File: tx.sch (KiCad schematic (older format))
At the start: 60 parts, among them T2 Transformer_1P_SS, U10 TLV2464CD, U11 SN74CBT3253

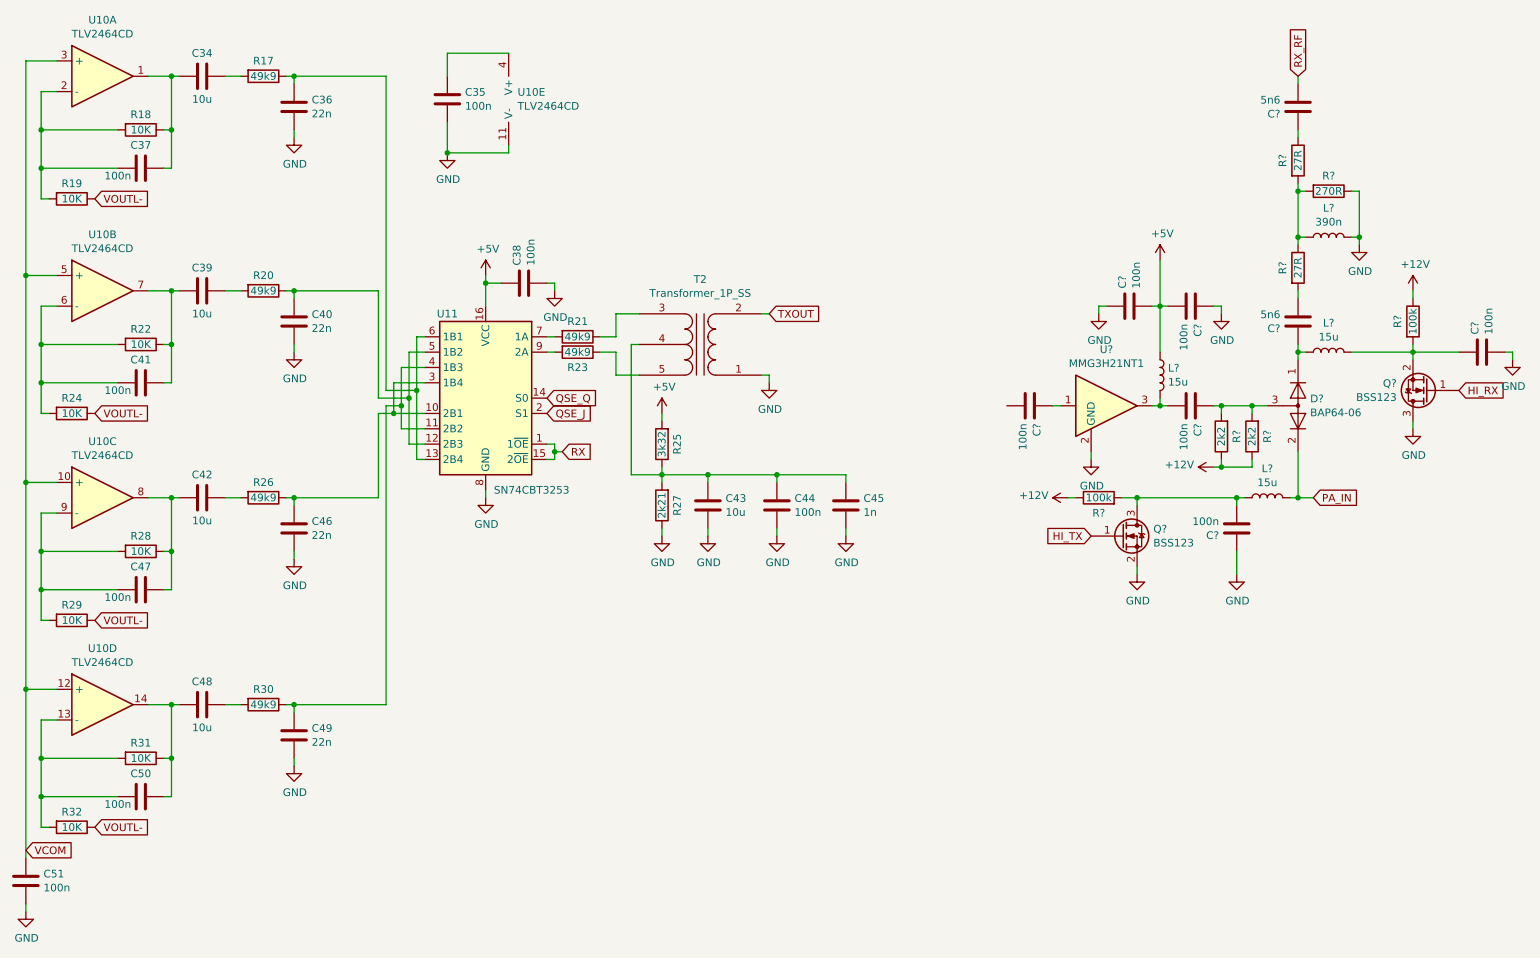
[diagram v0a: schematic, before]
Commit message: First layouting
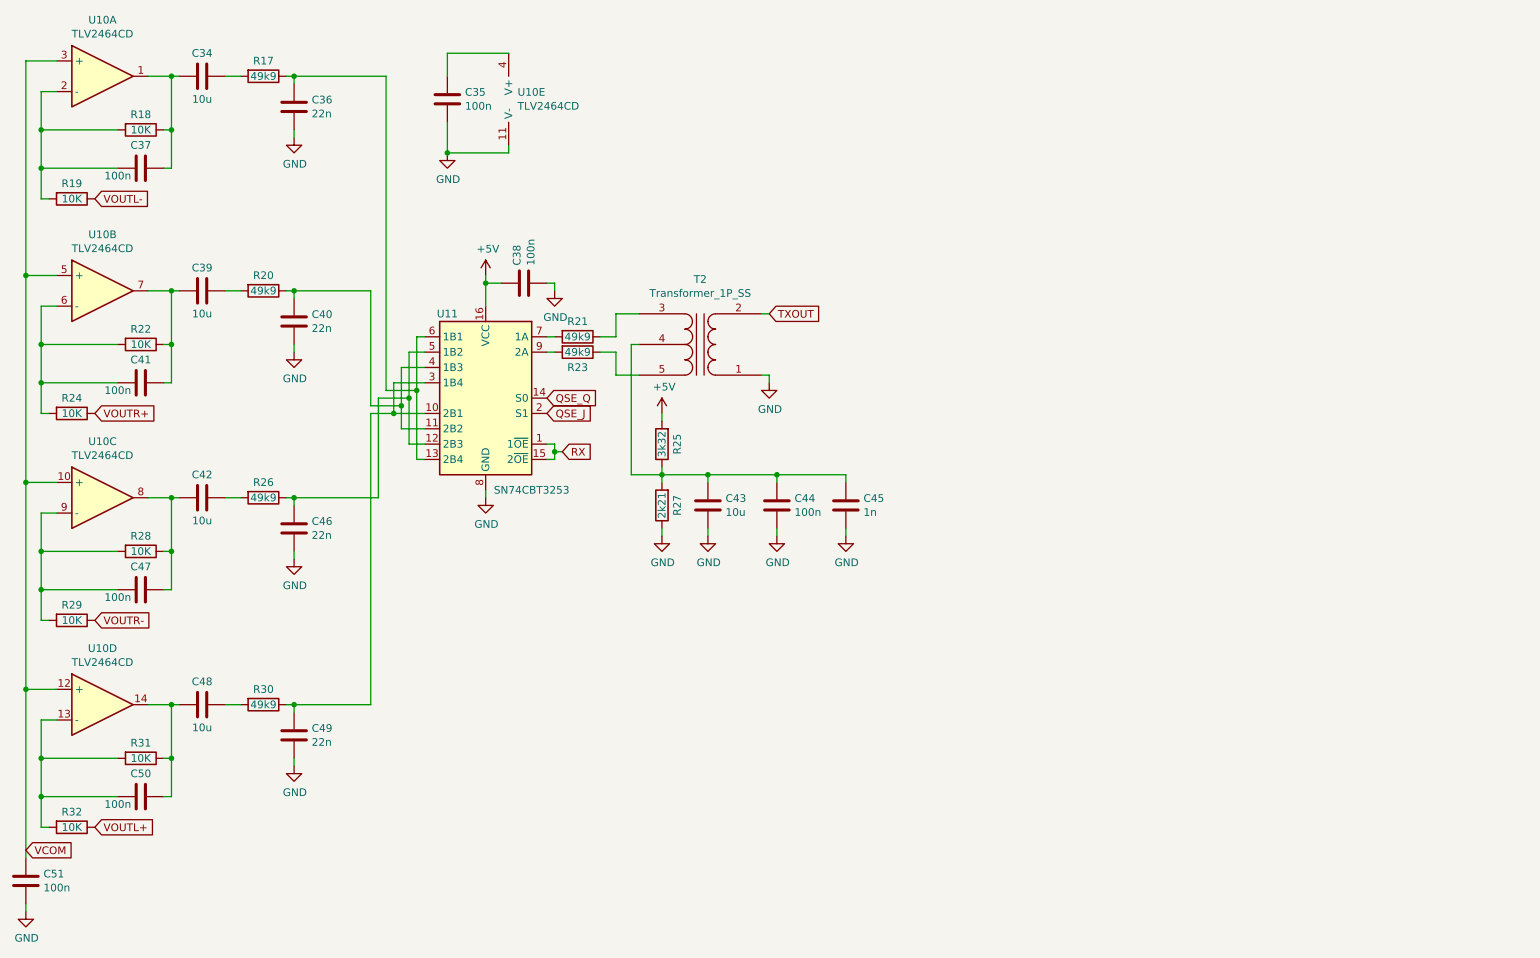
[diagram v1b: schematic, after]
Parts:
- removed C? (x6): 100n, Capacitor_SMD:C_0603_1608Metric, symbol DeltaSDR-rescue:C-Device-DeltaSDR-rescue
- removed C? (x2): 5n6, Capacitor_SMD:C_0603_1608Metric, symbol DeltaSDR-rescue:C-Device-DeltaSDR-rescue
- removed D?: BAP64-06, symbol Device:D_x2_ACom_KKA
- removed L? (x3): 15u, symbol Device:L
- removed L?: 390n, symbol Device:L
- removed Q? (x2): BSS123, Package_TO_SOT_SMD:SOT-23, symbol Transistor_FET:BSS123
- removed R? (x2): 2k2, Resistor_SMD:R_0603_1608Metric, symbol DeltaSDR-rescue:R-Device-DeltaSDR-rescue
- removed R? (x2): 100k, Resistor_SMD:R_0603_1608Metric, symbol DeltaSDR-rescue:R-Device-DeltaSDR-rescue
- removed R? (x2): 27R, Resistor_SMD:R_0603_1608Metric, symbol DeltaSDR-rescue:R-Device-DeltaSDR-rescue
- removed R?: 270R, Resistor_SMD:R_0603_1608Metric, symbol DeltaSDR-rescue:R-Device-DeltaSDR-rescue
- removed U?: MMG3H21NT1, Package_TO_SOT_SMD:SOT-89-3, symbol RF_Amplifier:SPF5189Z
- C43: footprint Capacitor_SMD:C_0603_1608Metric -> Capacitor_SMD:C_0805_2012Metric
- T2: footprint (none) -> Transformer_SMD:Transformer_MACOM_SM-22
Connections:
- net VOUTL-: no longer R24.1, R29.1, R32.1
- net at U11.10 (2B1), U11.3 (1B4): now also C49.1, R30.1; no longer C46.1, R26.1
- net at U11.11 (2B2), U11.4 (1B3): now also C40.1, R20.1; no longer C49.1, R30.1
- net at U11.12 (2B3), U11.5 (1B2): now also C46.1, R26.1; no longer C40.1, R20.1
- new net VOUTL+: R32.1
- new net VOUTR+: R24.1
- new net VOUTR-: R29.1
